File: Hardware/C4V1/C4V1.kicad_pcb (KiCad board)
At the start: 2 copper layers, 81 x 24 mm, 27 parts, among them IC1 W25Q16JVSNIQ, IC2 MB85RS256TYPNF-G-AWERE2, J1 48037-2100, J2 Prawo, J3 Lewo, U1 LDLN050PU33, U2 ESDALCL6-2SC6, U3 STM32G4A1KEU6, Y1 ECS-80-8-33Q-ADS-TR3

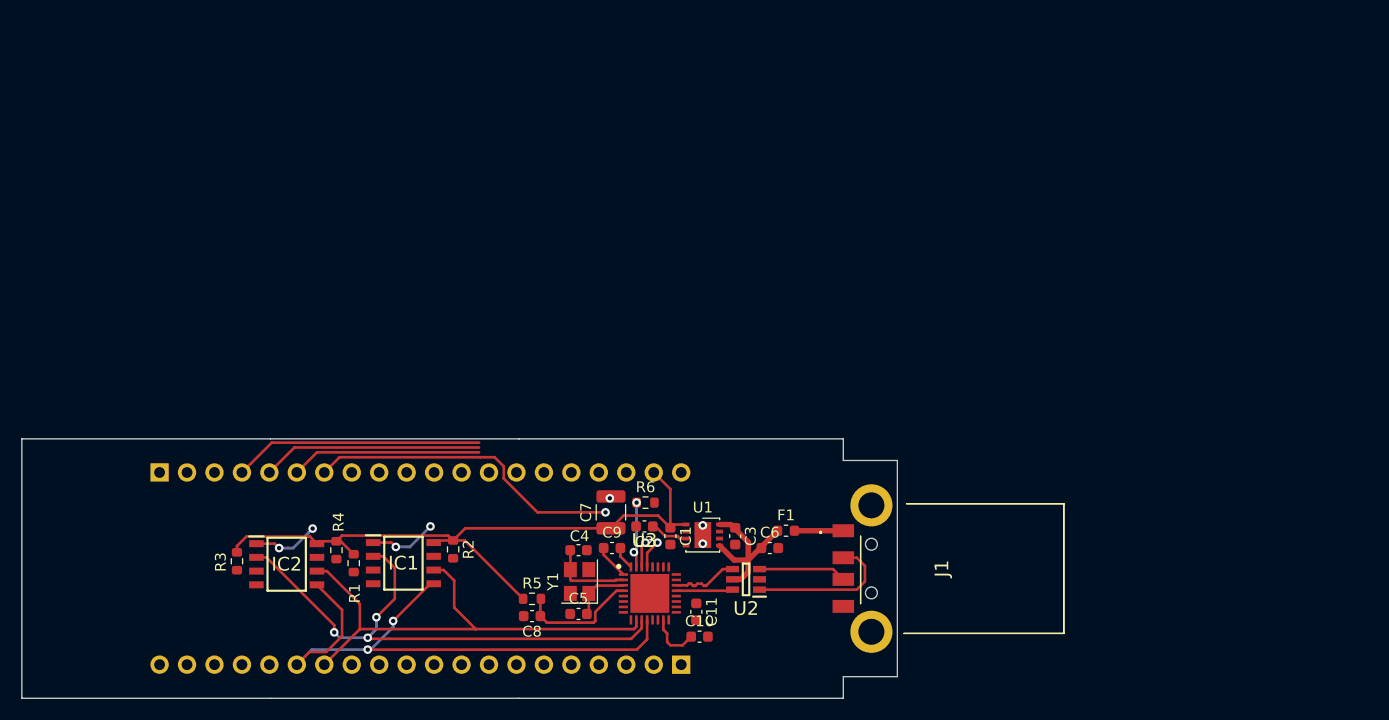
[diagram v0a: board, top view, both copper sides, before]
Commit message: Prawie ukończona płytka
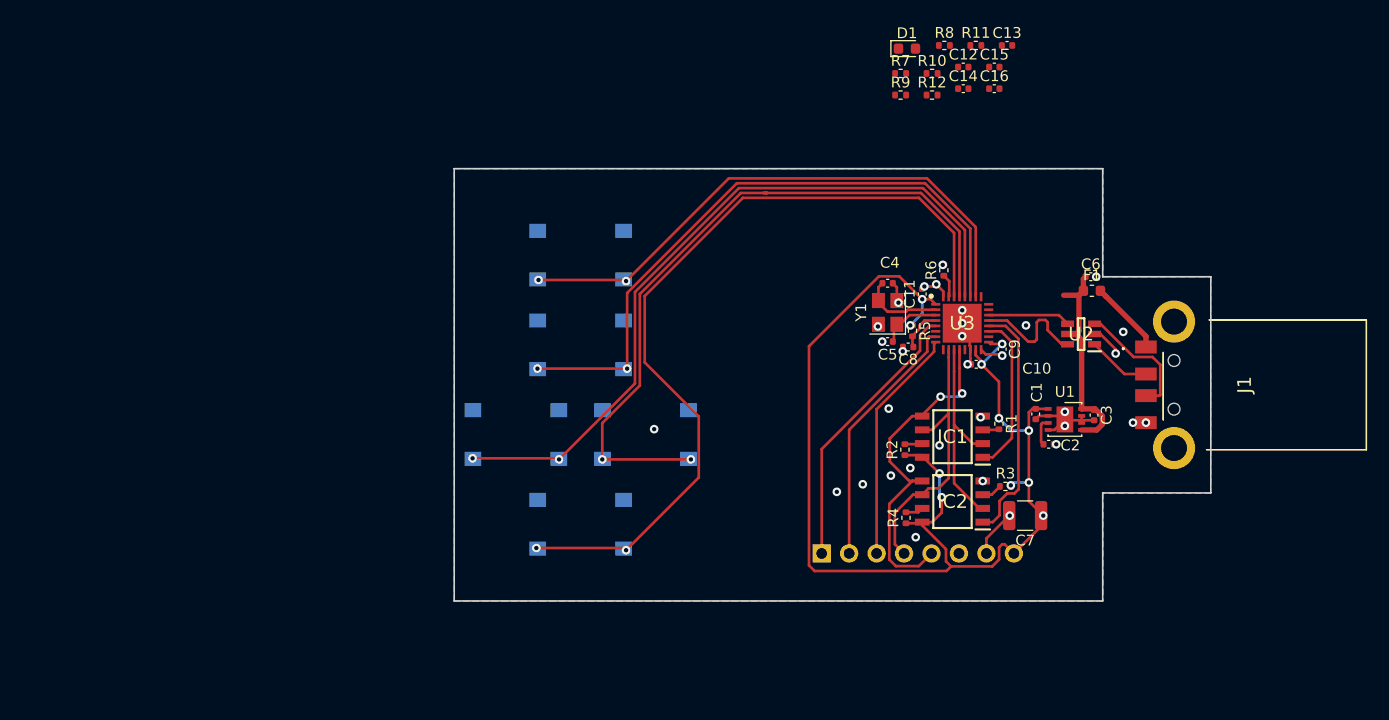
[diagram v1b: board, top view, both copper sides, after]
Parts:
- removed J3: Lewo, Connector_PinHeader_2.54mm:PinHeader_1x20_P2.54mm_Vertical
- added C12: 100n/X5R/10V, Capacitor_SMD:C_0402_1005Metric, F.Cu at (100.1, 86.6)
- added C13: 100n/X5R/10V, Capacitor_SMD:C_0402_1005Metric, F.Cu at (104.2, 84.6)
- added C14: 100n/X5R/10V, Capacitor_SMD:C_0402_1005Metric, F.Cu at (100.1, 88.6)
- added C15: 100n/X5R/10V, Capacitor_SMD:C_0402_1005Metric, F.Cu at (103.0, 86.6)
- added C16: 100n/X5R/10V, Capacitor_SMD:C_0402_1005Metric, F.Cu at (103.0, 88.6)
- added D1: LED, LED_SMD:LED_0603_1608Metric, F.Cu at (94.9, 84.9)
- added R10: 10k/5%/0.1W, Resistor_SMD:R_0402_1005Metric, F.Cu at (97.2, 87.2)
- added R11: 10k/5%/0.1W, Resistor_SMD:R_0402_1005Metric, F.Cu at (101.3, 84.6)
- added R12: 10k/5%/0.1W, Resistor_SMD:R_0402_1005Metric, F.Cu at (97.2, 89.2)
- added R7: /5%/0.1W, Resistor_SMD:R_0402_1005Metric, F.Cu at (94.3, 87.2)
- added R8: 10k/5%/0.1W, Resistor_SMD:R_0402_1005Metric, F.Cu at (98.3, 84.6)
- added R9: 10k/5%/0.1W, Resistor_SMD:R_0402_1005Metric, F.Cu at (94.3, 89.2)
- added SW1: SW_Push, Button_Switch_SMD:SW_Push_1P1T_NO_6x6mm_H9.5mm, B.Cu at (64.7, 128.9)
- added SW2: SW_Push, Button_Switch_SMD:SW_Push_1P1T_NO_6x6mm_H9.5mm, B.Cu at (64.7, 112.3)
- added SW3: SW_Push, Button_Switch_SMD:SW_Push_1P1T_NO_6x6mm_H9.5mm, B.Cu at (70.7, 120.6)
- added SW4: SW_Push, Button_Switch_SMD:SW_Push_1P1T_NO_6x6mm_H9.5mm, B.Cu at (58.7, 120.6)
- added SW5: SW_Push, Button_Switch_SMD:SW_Push_1P1T_NO_6x6mm_H9.5mm, B.Cu at (64.7, 104.0)
- C1, C10, C11, C2, C3, C4, C5, C6, C8, C9: footprint Capacitor_SMD:C_0603_1608Metric -> Capacitor_SMD:C_0402_1005Metric
- J2: value Prawo -> Conn_01x08_Male; footprint Connector_PinHeader_2.54mm:PinHeader_1x20_P2.54mm_Vertical -> Connector_PinHeader_2.54mm:PinHeader_1x08_P2.54mm_Vertical
- R1, R2, R3, R4, R5, R6: footprint Resistor_SMD:R_0603_1608Metric -> Resistor_SMD:R_0402_1005Metric
- moved R3 71.4 mm to (104.0, 125.4), turned to 180 degrees
- moved IC2 61.9 mm to (99.1, 126.8), turned to 180 degrees
- moved J2 61.7 mm to (87.0, 131.6)
- moved R1 61.1 mm to (103.4, 119.6)
- moved R4 52.8 mm to (94.8, 128.3), turned to 90 degrees
- moved IC1 52.1 mm to (99.1, 120.8), turned to 180 degrees
- moved R5 43.1 mm to (95.4, 111.0), turned to 270 degrees
- moved R2 42.8 mm to (94.7, 122.0), turned to 90 degrees
- moved C8 42.8 mm to (95.0, 112.5)
- moved C9 40.5 mm to (103.7, 112.7), turned to 270 degrees
- moved C6 38.9 mm to (111.9, 106.0)
- moved U2 38.4 mm to (111.0, 111.3)
- moved C7 38.3 mm to (105.8, 128.1), turned to 180 degrees
- moved U3 38.2 mm to (100.0, 110.3)
- moved C2 38.2 mm to (108.0, 121.5), turned to 0 degrees
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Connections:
- IC1 pad 1: FLASH_CS -> ~FLASH_CS
- IC2 pad 1: FRAM_CS -> ~FRAM_CS
- J2 pad 1: LEFT -> ~RES
- J2 pad 2: B -> DC
- J2 pad 3: GND -> ~CS
- J2 pad 4: DOWN -> CLK
- J2 pad 5: X -> MOSI
- J2 pad 6: RIGHT -> Net-(J2-Pad6)
- J2 pad 7: Y -> GND
- J2 pad 8: GND -> +3V3
- U3 pad 19: Net-(U3-Pad19) -> ~FLASH_CS
- U3 pad 20: Net-(U3-Pad20) -> ~FRAM_CS
- U3 pad 26: Net-(U3-Pad26) -> OK
- U3 pad 28: X -> RIGHT
- U3 pad 29: RIGHT -> LEFT
- U3 pad 30: Y -> UP
- U3 pad 5: Net-(U3-Pad5) -> ~RES
- U3 pad 7: Net-(U3-Pad7) -> DC
- U3 pad 8: Net-(U3-Pad8) -> ~CS
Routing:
- net UP: track 0.00 -> 76.4 mm, vias 0 -> 2
- net LEFT: track 0.00 -> 66.3 mm, vias 0 -> 2
- net OK: track 0.00 -> 52.7 mm, vias 0 -> 2
- net RIGHT: track 20.3 -> 68.7 mm, vias 1 -> 2
- net +3V3: track 71.3 -> 109.7 mm, vias 0 -> 11
- net DOWN: track 23.1 -> 59.3 mm, vias 0 -> 2
- net Y: track 31.8 -> 0.00 mm, vias 2 -> 0
- net MISO: track 50.3 -> 19.3 mm, vias 3 -> 0
- net GND: track 2.15 -> 28.4 mm, vias 3 -> 32
- net ~RES: track 0.00 -> 25.8 mm
- net DC: track 0.00 -> 23.7 mm
- net MOSI: track 55.3 -> 32.2 mm
- net ~FRAM_CS: track 0.00 -> 22.5 mm
- net ~CS: track 0.00 -> 21.8 mm
- net CLK: track 46.1 -> 25.4 mm
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- added copper zone on B.Cu, net GND
- added copper zone on F.Cu, net GND
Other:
- board size 81 x 24 mm -> 70 x 40 mm
